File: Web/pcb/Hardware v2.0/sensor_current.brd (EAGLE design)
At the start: 30.5 x 14.9 mm, 7 parts

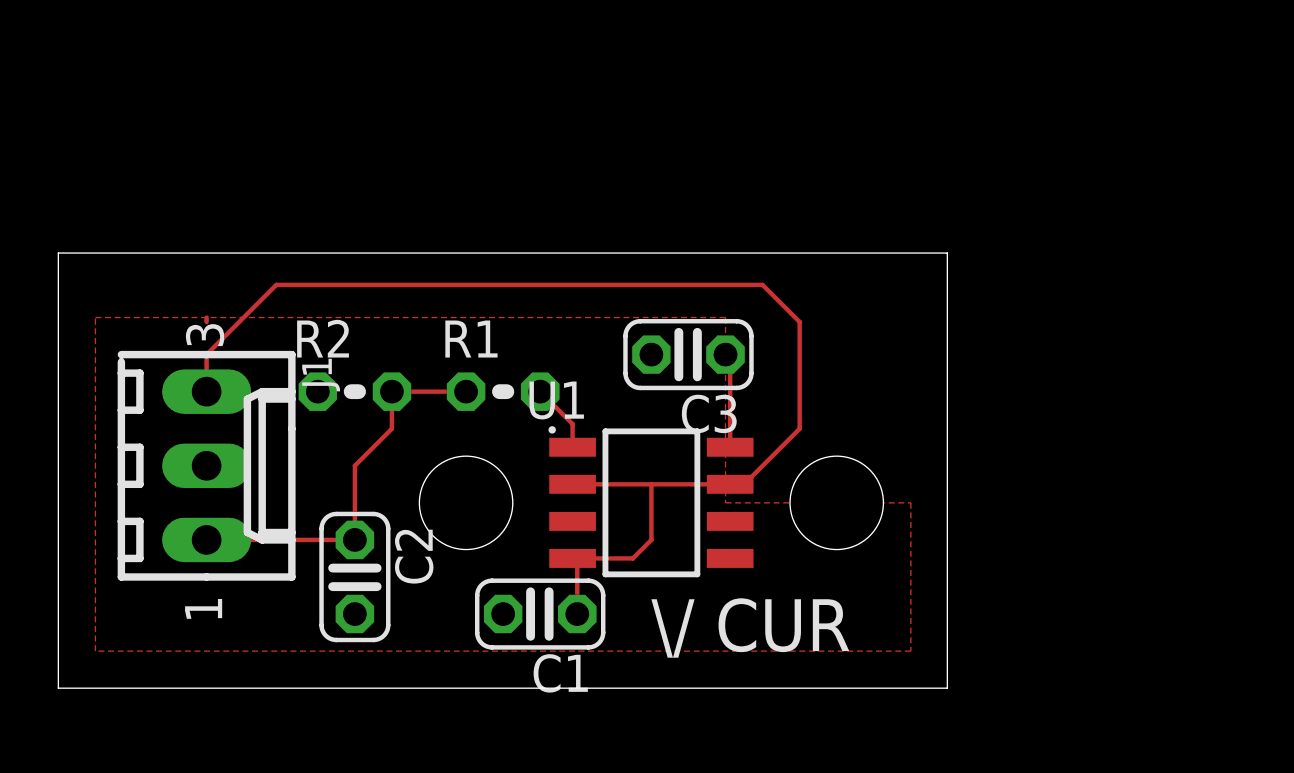
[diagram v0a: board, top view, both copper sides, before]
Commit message: updates
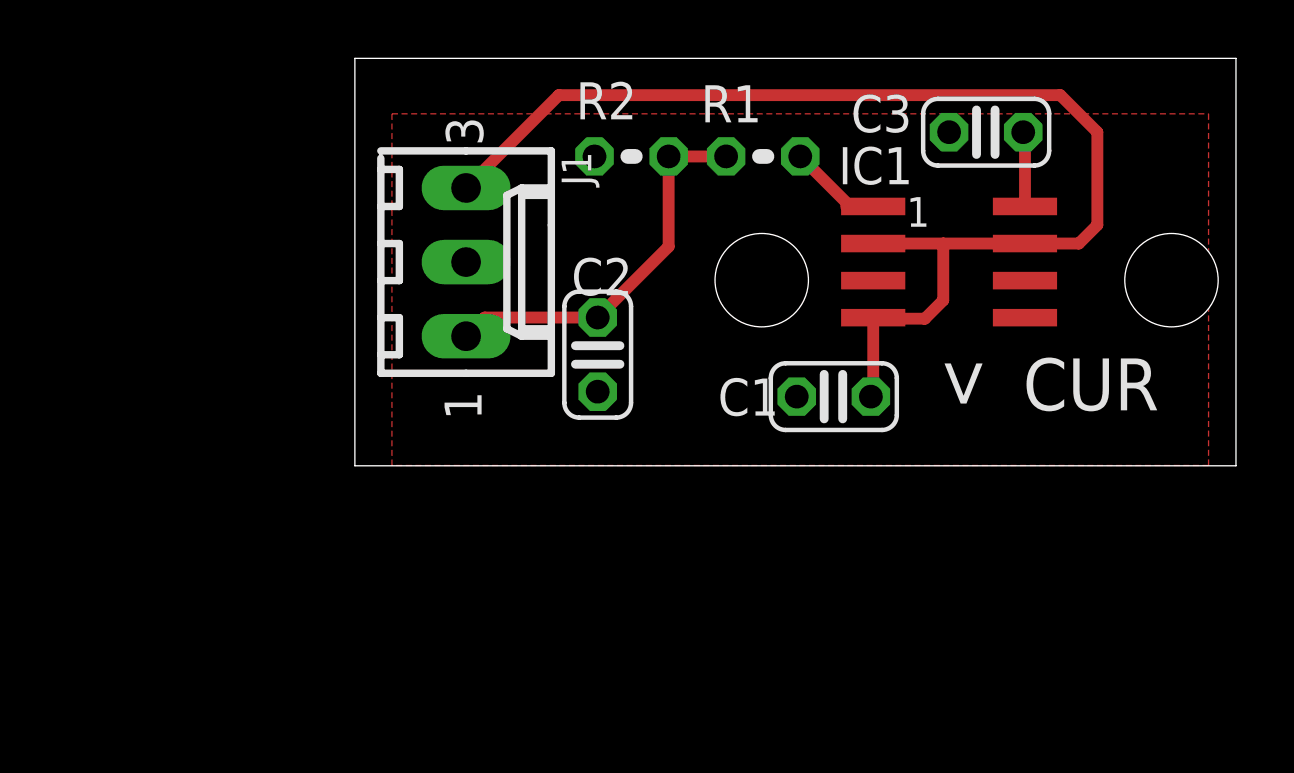
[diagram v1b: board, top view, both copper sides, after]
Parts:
- removed U1: (no value), MLX91208:SOIC127P602X179-8N
- added IC1: MLX91205, melexis:SO-08
- C1: value 1uF -> 1µ
- J1: value (none) -> 22-27-2031-03
- moved C3 12.7 mm to (21.6, 11.4)
- moved C1 12.5 mm to (16.4, 2.37)
- moved R2 12.4 mm to (9.48, 10.6)
- moved R1 12.0 mm to (14.0, 10.6)
- moved J1 11.3 mm to (3.81, 6.98)
- moved C2 11.3 mm to (8.32, 3.81)
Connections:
- removed net N$3 (its old number): R1.2, U1.1
- new net N$2: C3.1, IC1.8
- net GND: now also IC1.5, IC1.6; no longer U1.5, U1.6
- net N$1: now also IC1.1, R1.2; no longer C3.1, U1.8
- net VCC: now also IC1.2, IC1.4, IC1.7; no longer U1.2, U1.4, U1.7
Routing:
- net N$2: track 0.00 -> 3.05 mm
- net N$3 (its old number): track 2.36 -> 0.00 mm
- net N$1: track 3.24 -> 4.14 mm
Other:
- board size 30.5 x 14.9 mm -> 30.2 x 14 mm
- board text added: "1"
- board text added: "<"
- board text added: "CUR"
- board text removed: "\\/ CUR"

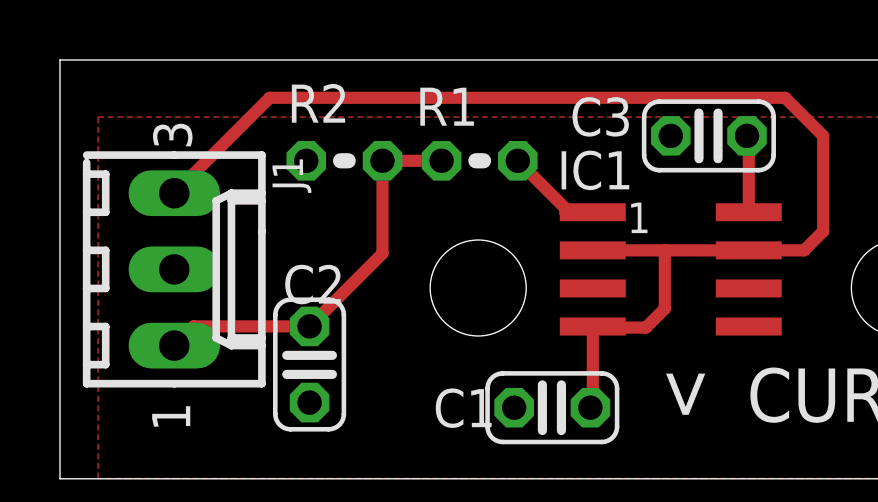
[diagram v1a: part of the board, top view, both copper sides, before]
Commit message: software updates
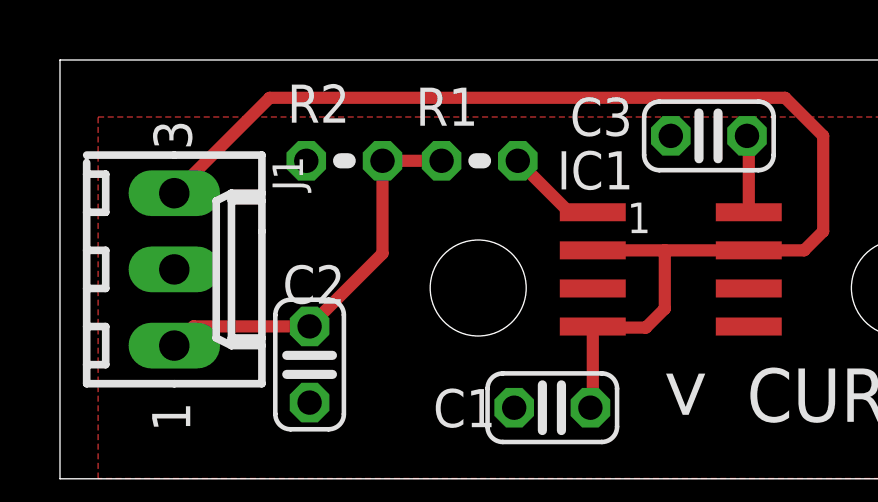
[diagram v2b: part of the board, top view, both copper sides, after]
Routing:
- net N$1: track 4.14 -> 3.21 mm
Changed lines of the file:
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@@
 <?xml version="1.0" encoding="utf-8"?>
 <!DOCTYPE eagle SYSTEM "eagle.dtd">
-<eagle version="9.1.3">
+<eagle version="9.2.2">
 <drawing>
 <settings>
@@
 <attribute name="VALUE" x="22.9" y="13.97" size="1.27" layer="27" rot="R180"/>
 </element>
-<element name="R1" library="rcl" package="0204V" value="1k2" x="13.99" y="10.6"/>
+<element name="R1" library="rcl" package="0204V" value="1k2" x="13.99" y="10.6" smashed="yes">
+<attribute name="NAME" x="11.8564" y="11.7684" size="1.27" layer="25" ratio="10"/>
+<attribute name="VALUE" x="11.8564" y="8.2886" size="1.27" layer="27" ratio="10"/>
+</element>
 <element name="R2" library="rcl" package="0204V" value="3k3" x="9.48" y="10.6" smashed="yes">
 <attribute name="NAME" x="7.575" y="11.87" size="1.27" layer="25"/>
 <attribute name="VALUE" x="8.845" y="8.06" size="1.27" layer="27"/>
 </element>
-<element name="J1" library="con-molex" package="6410-03" value="22-27-2031-03" x="3.81" y="6.98" rot="R270">
+<element name="J1" library="con-molex" package="6410-03" value="22-27-2031-03" x="3.81" y="6.98" smashed="yes" rot="R270">
 <attribute name="MF" value="" x="-13.97" y="-12.07" size="1.778" layer="27" rot="R270" display="off"/>
 <attribute name="MPN" value="" x="-13.97" y="-12.07" size="1.778" layer="27" rot="R270" display="off"/>
+<attribute name="NAME" x="7.0851" y="10.7631" size="1.016" layer="25" ratio="10" rot="R270"/>
 <attribute name="OC_FARNELL" value="unknown" x="-13.97" y="-12.07" size="1.778" layer="27" rot="R270" display="off"/>
 <attribute name="OC_NEWARK" value="unknown" x="-13.97" y="-12.07" size="1.778" layer="27" rot="R270" display="off"/>
+<attribute name="VALUE" x="-0.7889" y="10.7631" size="0.8128" layer="27" ratio="10" rot="R270"/>
 </element>
 </elements>
@@
 <contactref element="IC1" pad="1"/>
 <contactref element="R1" pad="2"/>
-<wire x1="16.835" y1="8.885" x2="17.76" y2="8.885" width="0.4064" layer="1"/>
 <wire x1="15.26" y1="10.6" x2="16.975" y2="8.885" width="0.4064" layer="1"/>
 <wire x1="16.975" y1="8.885" x2="17.76" y2="8.885" width="0.4064" layer="1"/>
